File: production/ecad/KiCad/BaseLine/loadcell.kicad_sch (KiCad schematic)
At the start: 12 parts, among them J1 LoadCellConnector, U1 ADS122C04IPW, U6 LM741, U7 ADS1231IDR

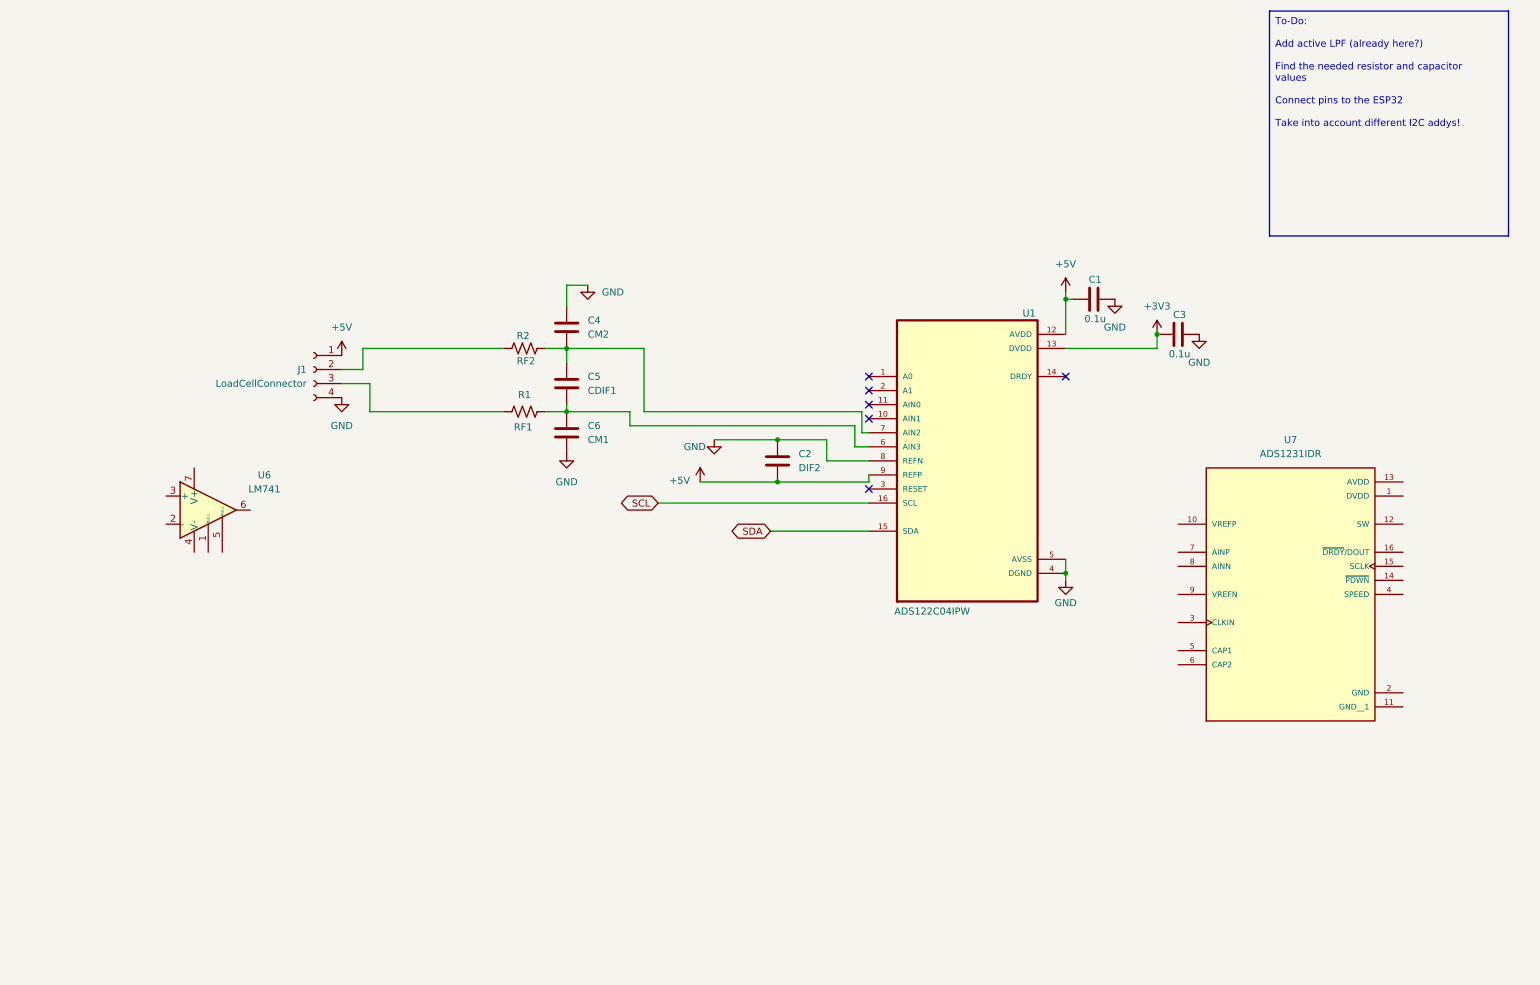
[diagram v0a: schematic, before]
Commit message: Load Cell changes
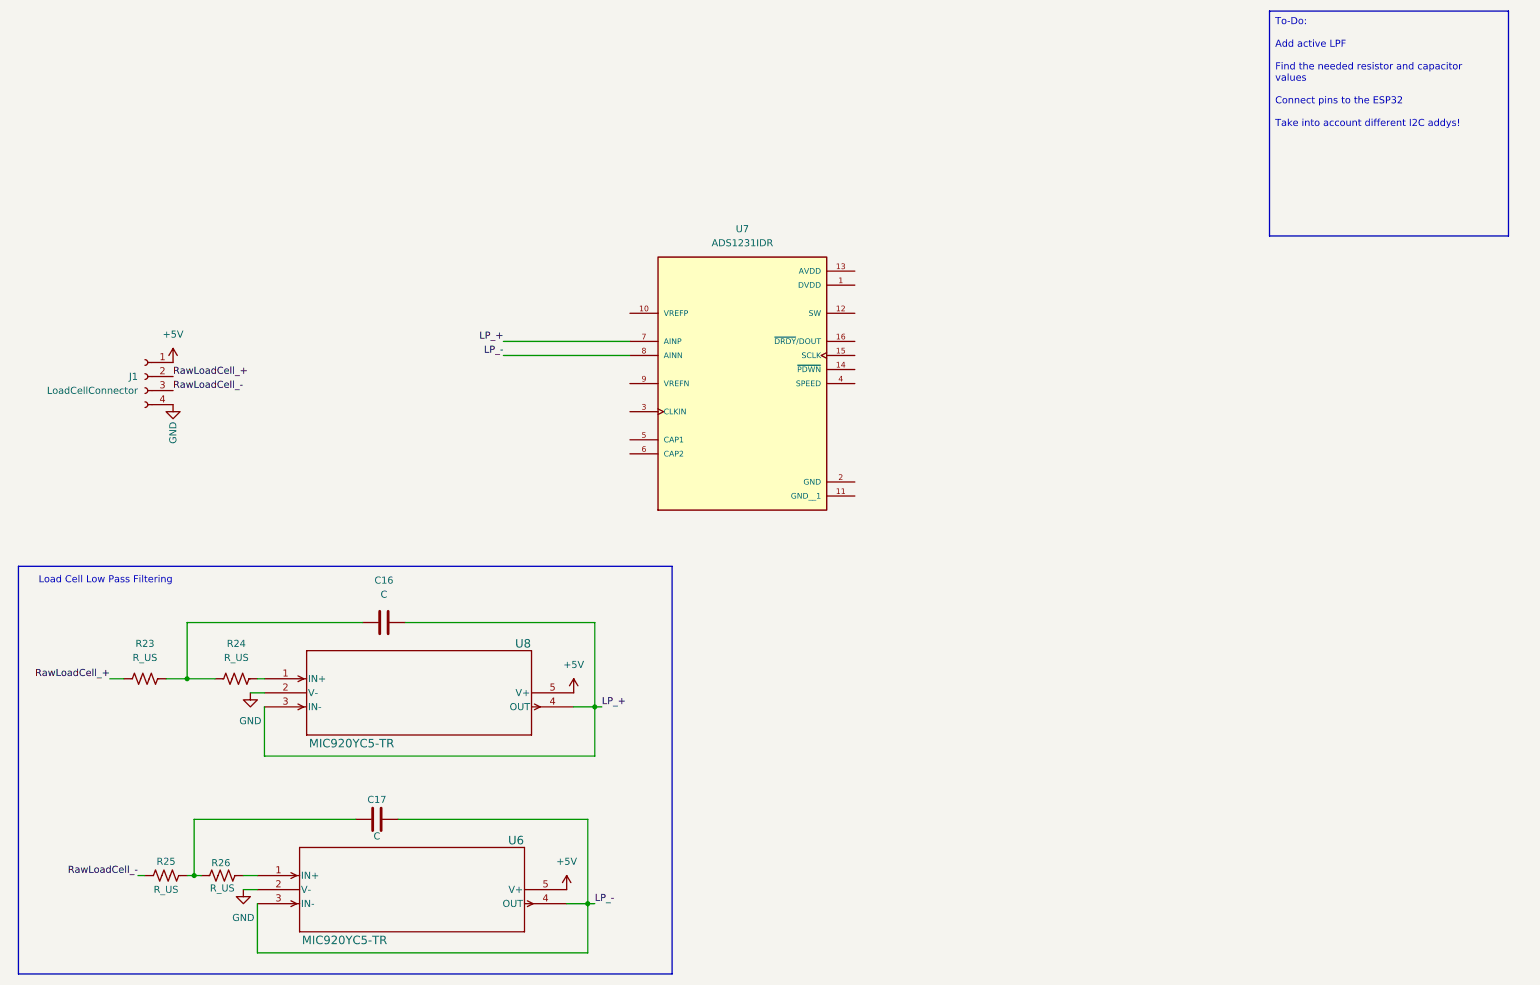
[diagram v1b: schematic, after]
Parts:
- removed C1, C3: 0.1u, symbol Device:C
- removed C2: DIF2, symbol Device:C
- removed C4: CM2, symbol Device:C
- removed C5: CDIF1, symbol Device:C
- removed C6: CM1, symbol Device:C
- removed R1: RF1, symbol Device:R_US
- removed R2: RF2, symbol Device:R_US
- removed U1: ADS122C04IPW, ADS122C04IPW:SOP65P640X120-16N, symbol ADS122C04IPW:ADS122C04IPW
- removed U6: LM741, symbol Amplifier_Operational:LM741
- added C16, C17: C, symbol Device:C
- added R23, R24, R25, R26: R_US, symbol Device:R_US
- added U6, U8: MIC920YC5-TR, SC-70_C5_MCH, symbol 2024-10-08_01-43-59:MIC920YC5-TR
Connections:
- net +5V: now also U6.5 (V+), U8.5 (V+)
- net GND: now also U6.2 (V-), U8.2 (V-)
- net RawLoadCell_-: now reaches J1.3 (Pin_3)
- net RawLoadCell_-: now also R25.2
- net RawLoadCell_+: now reaches J1.2 (Pin_2)
- net RawLoadCell_+: now also R23.2
- net LP_+: now reaches U7.7 (AINP)
- net LP_+: now also C16.2, U8.3 (IN-), U8.4 (OUT)
- net LP_-: now reaches U7.8 (AINN)
- net LP_-: now also C17.2, U6.3 (IN-), U6.4 (OUT)
- new net: R26.1, U6.1 (IN+)
- new net: C17.1, R25.1, R26.2
- new net: C16.1, R23.1, R24.2
- new net: R24.1, U8.1 (IN+)
- no-connect marks 6 -> 0
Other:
- note added: "Load Cell Low Pass Filtering"
- moved on the sheet: J1, U7
